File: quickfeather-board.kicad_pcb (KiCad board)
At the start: 4 copper layers, 58.4 x 22.9 mm, 101 parts, among them IC1 EOS-S3-QFN, J1 61300211121, J2 1x12_pinhead, J3 1x16_pinhead, J4 S2B-PH-SM4-TB_LF__SN_, J5 0473460001, J6 FTSH-105-01-L-DV-K, J7 61300211121, J8 2x8_pinhead, M1 mounting_pad, M2 mounting_pad, M3 mounting_pad, M4 mounting_pad, Q1 NX3008CBKV, Q2 2N7002PV, Q3 2N7002PV, Q4 DMG1012T-7, U1 TPS62821DLCR, U2 MCP73831T-2ACI_OT, U3 GD25Q16CWIGR, U4 DPS310, U5 MC3635, X1 ECS-_327-12_5-34B-TR

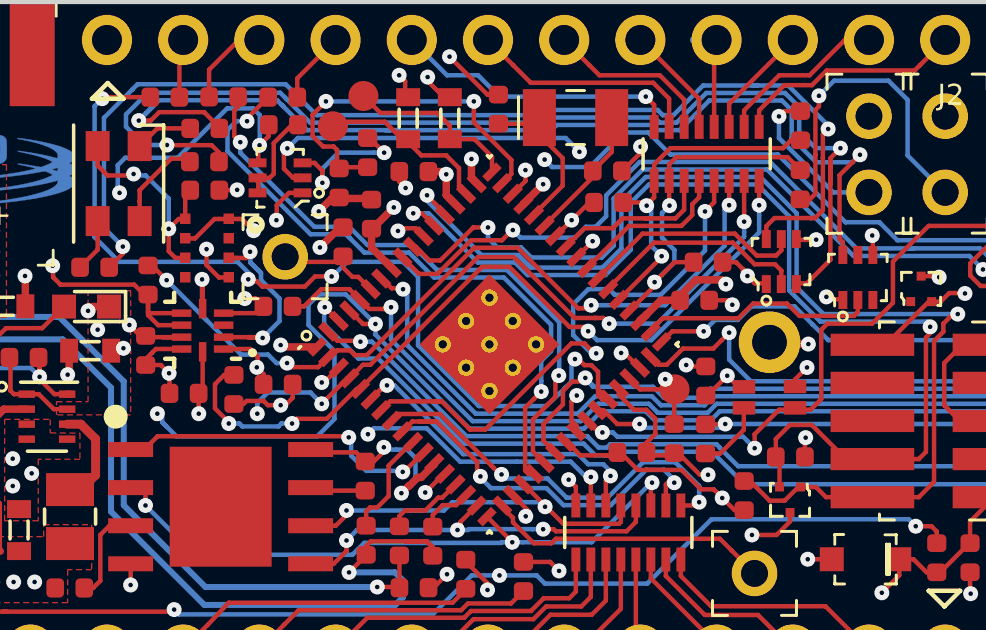
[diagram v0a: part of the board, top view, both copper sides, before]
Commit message: Update docs for release 1.2.1
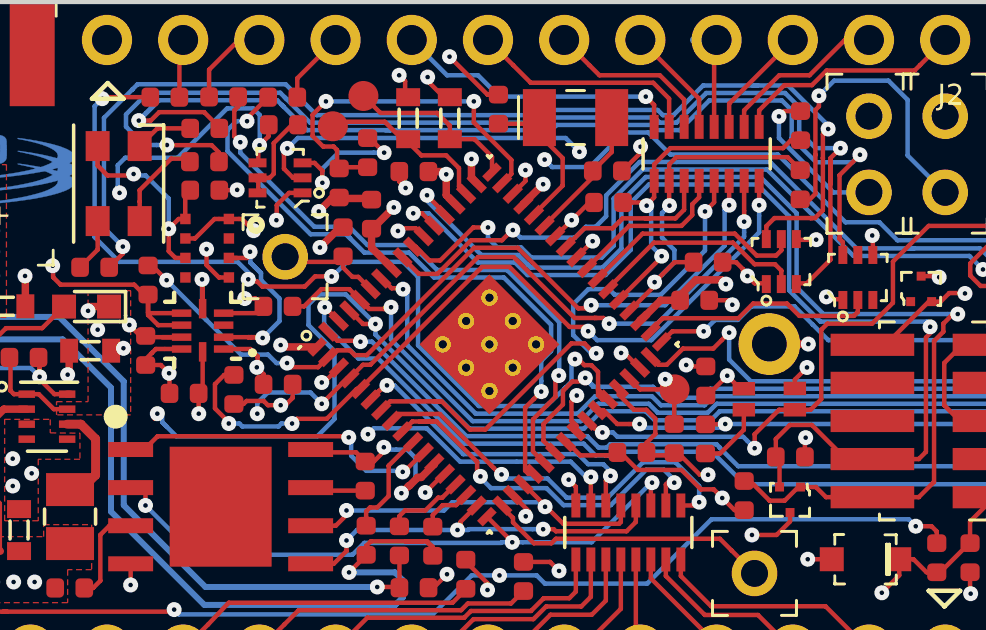
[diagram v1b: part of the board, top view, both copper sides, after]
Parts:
- moved MIC1 0.06 mm to (161.7, 105.0)
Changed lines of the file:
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@@
   (layers
     (0 Top signal)
-    (1 In1.Cu signal hide)
-    (2 In2.Cu mixed hide)
-    (31 Bottom signal hide)
+    (1 In1.Cu signal)
+    (2 In2.Cu mixed)
+    (31 Bottom signal)
     (32 B.Adhes user hide)
     (33 F.Adhes user hide)
@@
     (42 Eco1.User user hide)
     (43 Eco2.User user hide)
-    (44 Edge.Cuts user)
+    (44 Edge.Cuts user hide)
     (45 Margin user hide)
     (46 B.CrtYd user hide)
@@
   )
   (module quickfeather-board-footprints:IM69D130 (layer Top)
-    (at 161.6953 104.9267)
+    (at 161.69 104.99)
     (attr smd)
-    (fp_text reference MIC1 (at 0.41 -3.29) (layer F.SilkS) hide
-      (effects (font (size 1 1) (thickness 0.15)))
+    (fp_text reference MIC1 (at -2.18 0.34 -270) (layer F.SilkS) hide
+      (effects (font (size 0.7 0.7) (thickness 0.15)))
     )
     (fp_text value IM69D130 (at 1.95 -2.01) (layer F.Fab) hide
@@
   )
   (module quickfeather-board-footprints:PG-VLGA-8-2 (layer Top)
-    (at 142.9453 101.7767)
+    (at 142.95 101.785)
     (attr smd)
-    (fp_text reference U4 (at -3.5 1) (layer F.SilkS) hide
+    (fp_text reference U4 (at 0.8 -0.05) (layer F.SilkS) hide
+      (effects (font (size 0.7 0.7) (thickness 0.15)))
+    )
+    (fp_text value DPS310 (at -0.05 -0.55) (layer F.Fab) hide
       (effects (font (size 1 1) (thickness 0.15)))
     )
-    (fp_text value DPS310 (at -1.32 -2.328) (layer F.Fab) hide
-      (effects (font (size 1 1) (thickness 0.15)))
-    )
